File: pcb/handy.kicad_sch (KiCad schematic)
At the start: 23 parts, among them J1 JST-SH 1x4, J2 JST-SH 1x4, J3 Conn_01x03_Pin, U1 TCA9548ARGER, U2 AS5600L-ASOM, U3 AS5600L-ASOM, U4 DRV8830DGQR, U5 ICM-42670-P

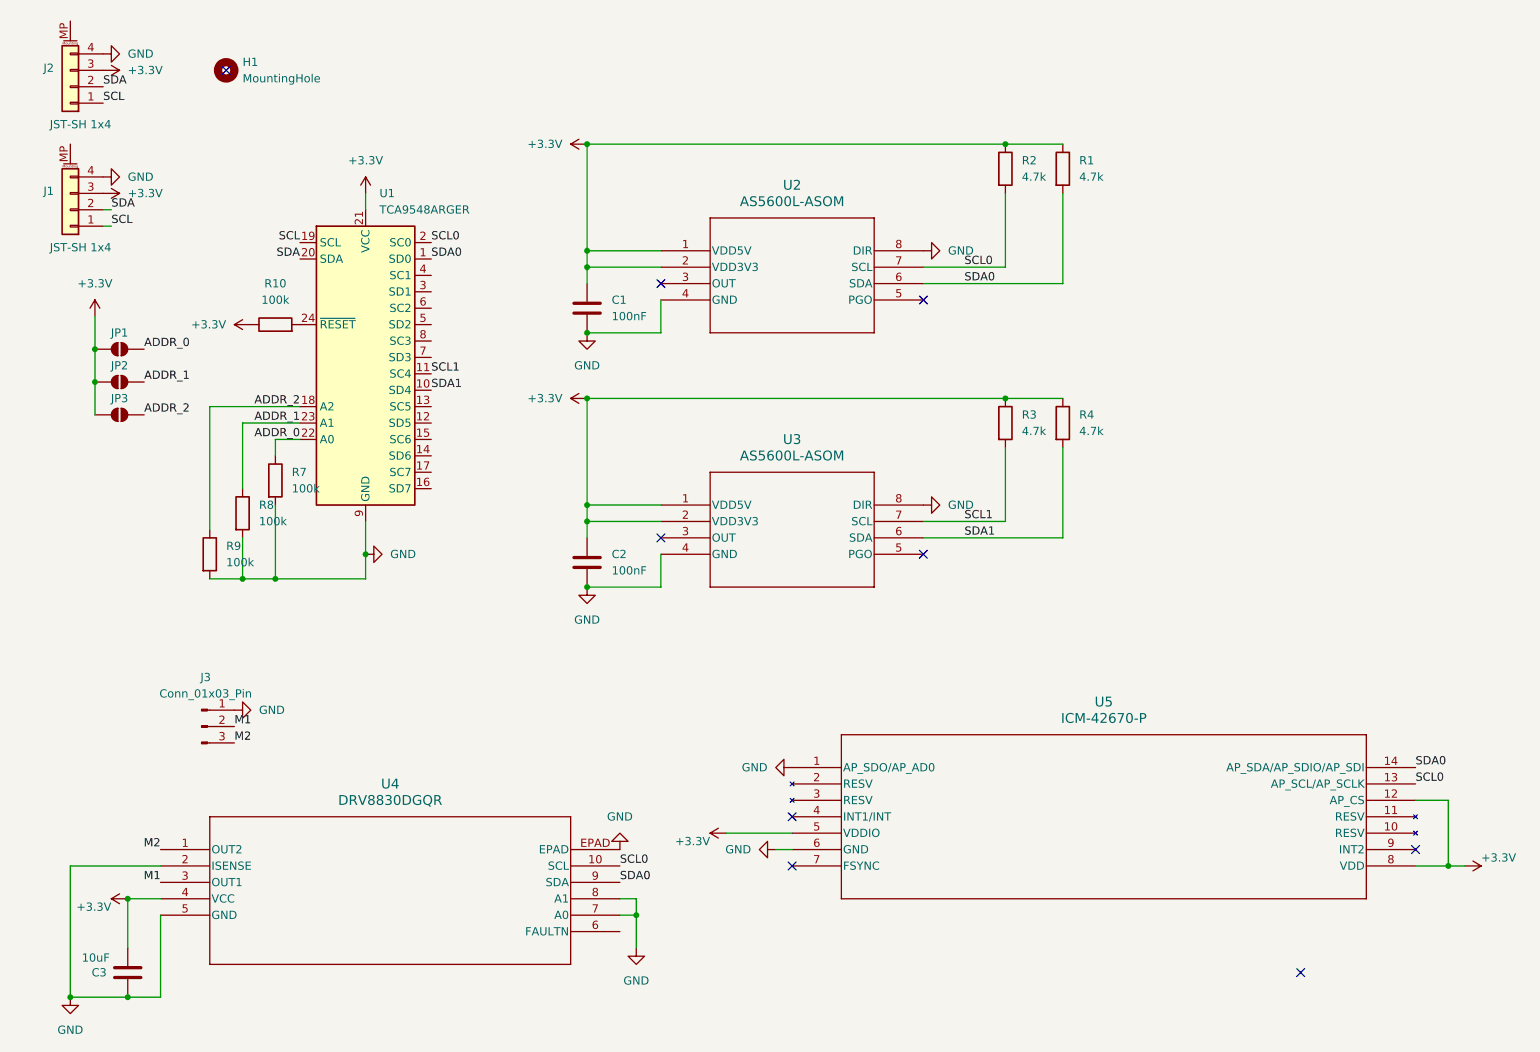
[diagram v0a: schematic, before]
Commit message: figure graphing
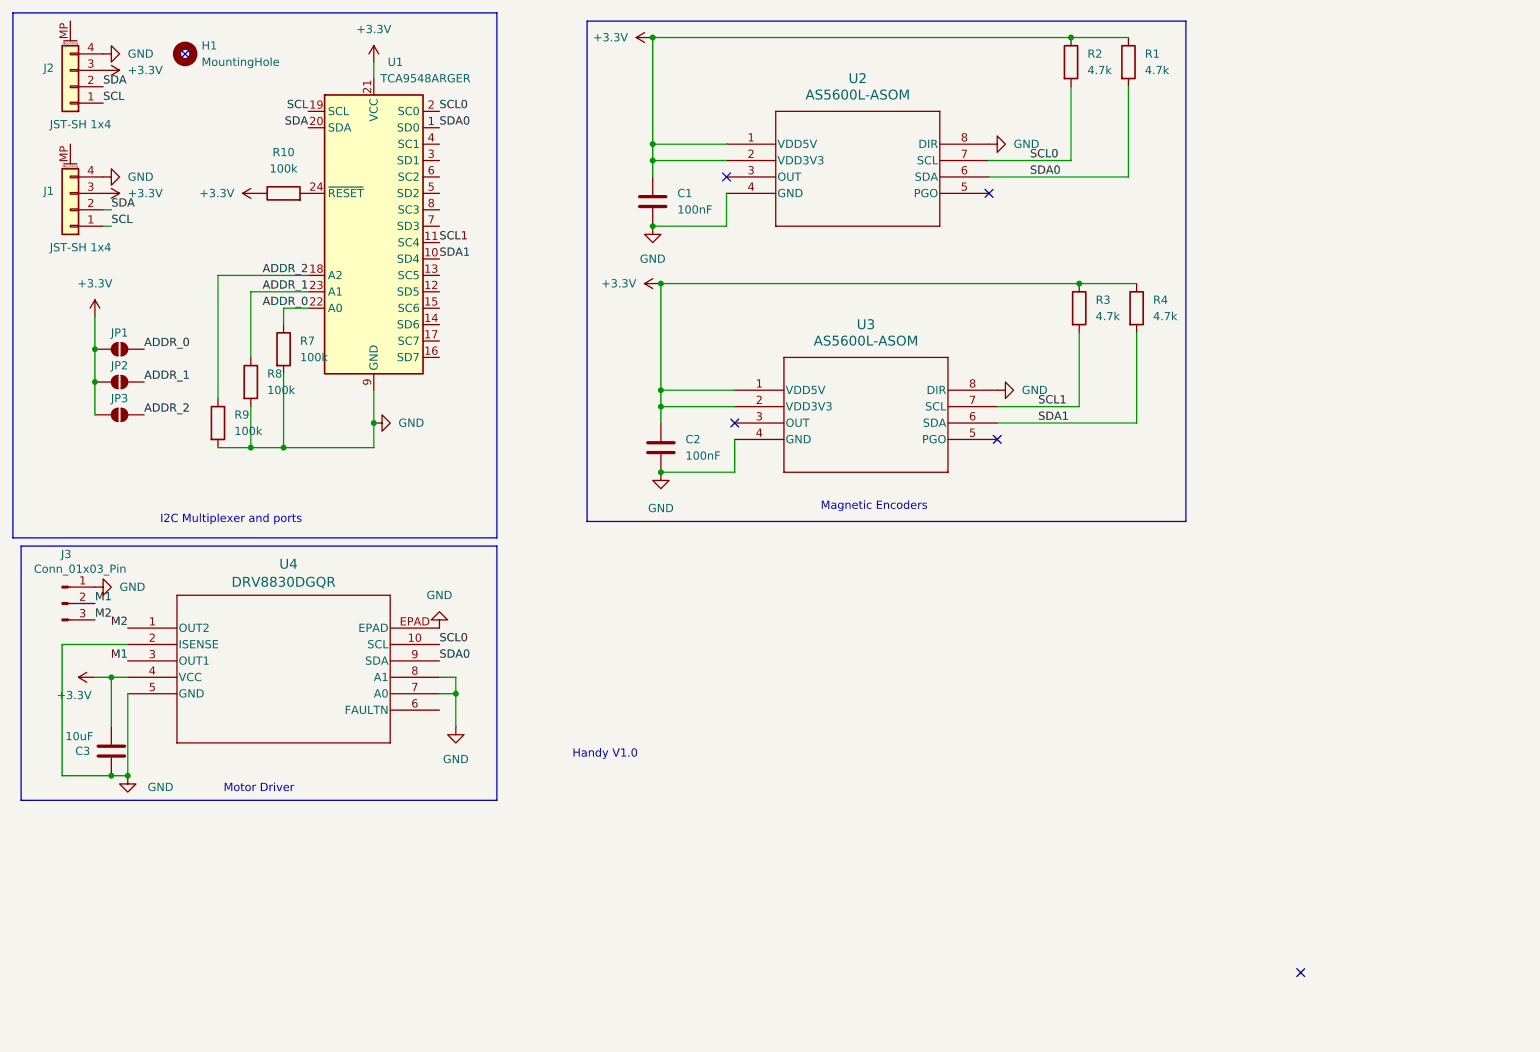
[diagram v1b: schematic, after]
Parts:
- removed U5: ICM-42670-P, ICM42670:LGA14_2.5X3X0.76_IVS, symbol icm42670:ICM-42670-P
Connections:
- no-connect marks 9 -> 6
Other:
- note added: "Handy V1.0"
- note added: "I2C Multiplexer and ports"
- note added: "Magnetic Encoders"
- note added: "Motor Driver"
- moved on the sheet: C1, C2, C3, H1, J3, R1, R10, R2, R3, R4, R7, R8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
